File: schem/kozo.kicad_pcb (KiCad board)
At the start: 2 copper layers, 40.6 x 22.9 mm, 22 parts, among them IC1 MSP430G2231IPW14, IC2 L78L33_SOT89, J1 Conn_01x02, J2 Conn_01x04, J3 Conn_01x03, J4 Conn_01x06, X1 Conn_01x03

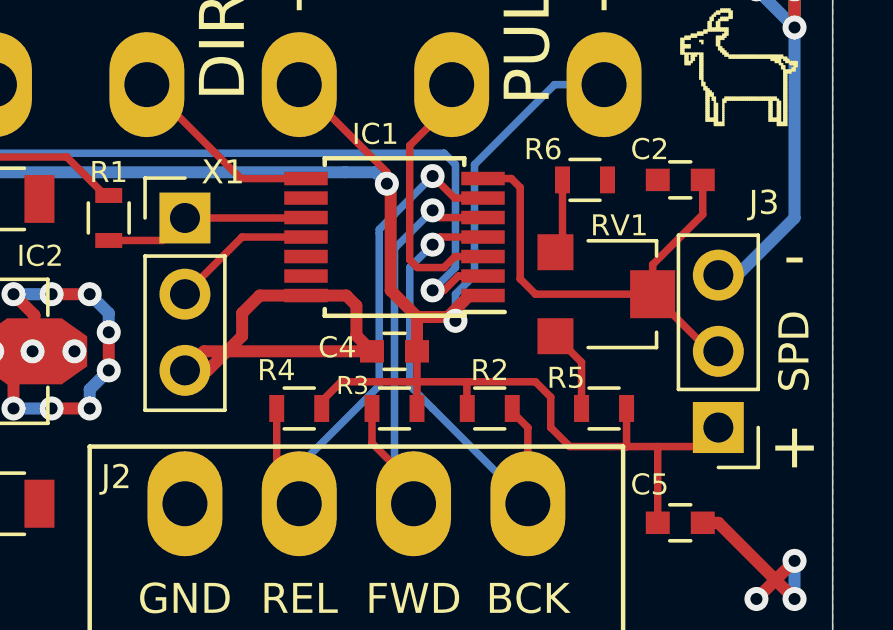
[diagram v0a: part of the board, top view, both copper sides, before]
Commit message: mask debug
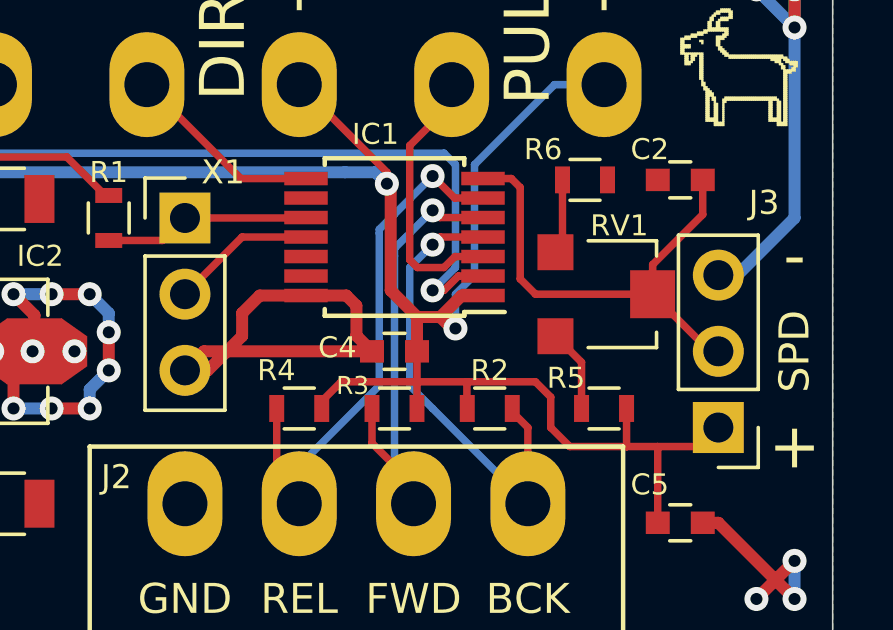
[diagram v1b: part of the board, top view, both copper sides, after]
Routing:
- net +3V3: track 77.0 -> 78.3 mm
